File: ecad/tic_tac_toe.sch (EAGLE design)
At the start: 36 parts, among them J1 PJ-102AH, U2 NCP1117ST50T3G, U3 ATMEGA8U2-AU, Y1 ECS-160-12-33-AGN-TR

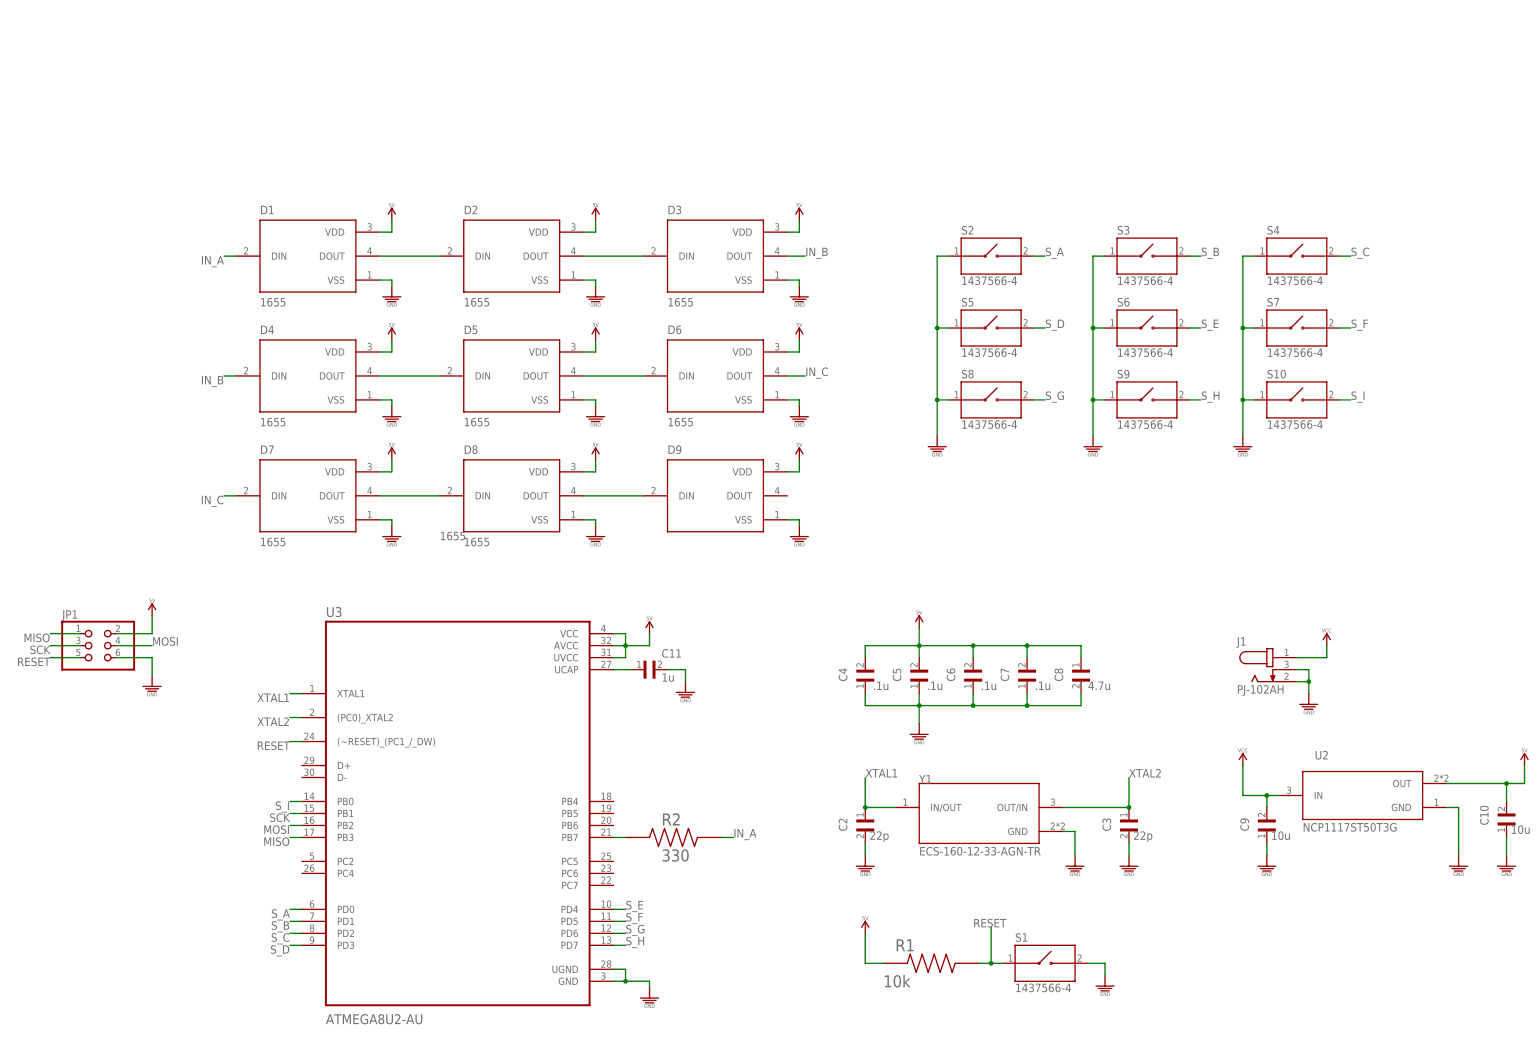
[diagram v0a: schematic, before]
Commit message: ecad, gerbers
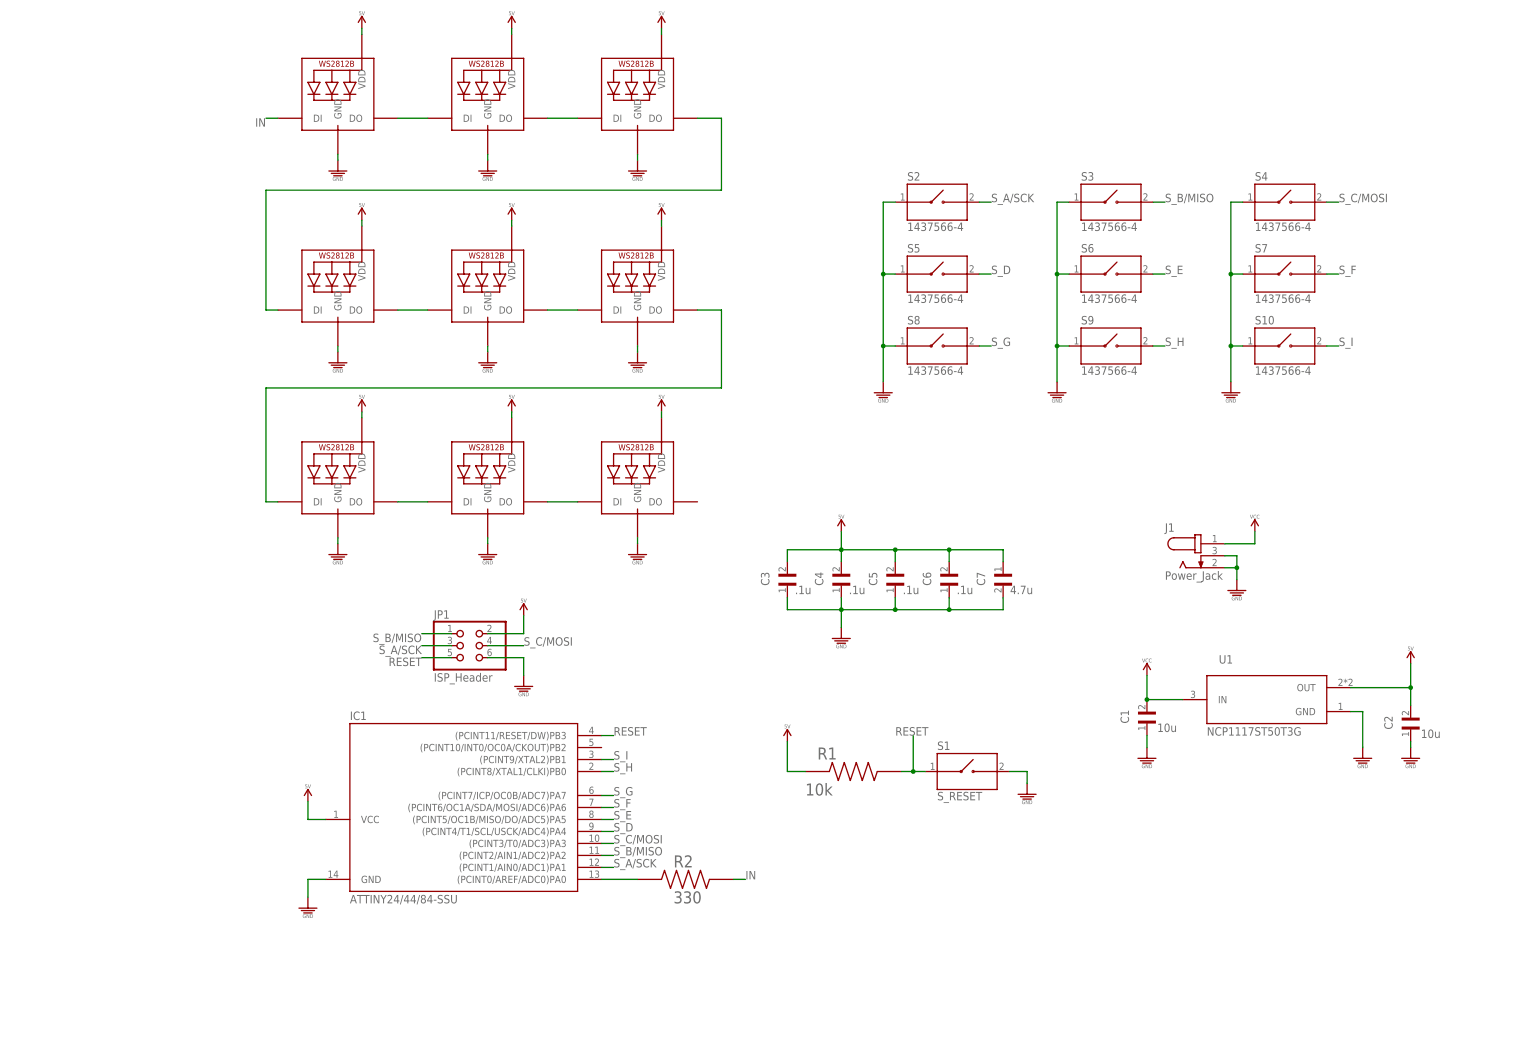
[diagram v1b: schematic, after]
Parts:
- removed C10, C9: 10u, TAJR106M006R:TAJR106M006R
- removed C11: 1u, GRM216R61E105KA12D:GRM216R61E105KA12D
- removed C8: 4.7u, CL21A475KAQNNNE:CL21A475KAQNNNE
- removed D1, D2, D3, D4, D5, D6, D7, D8, D9: 1655, 1655:1655
- removed U2: NCP1117ST50T3G, NCP1117ST50T3G:NCP1117ST50T3G
- removed U3: ATMEGA8U2-AU, ATMEGA8U2-AU:ATMEGA8U2-AU
- removed Y1: ECS-160-12-33-AGN-TR, ECS-160-12-33-AGN-TR:ECS-160-12-33-AGN-TR
- added C1: 10u, TAJR106M006R (1):TAJR106M006R
- added IC1: ATTINY24/44/84-SSU, attiny24_44_84:ATTINY24/44/84-SSU
- added LED1, LED2, LED3, LED4, LED5, LED6, LED7, LED8, LED9: MICROBUILDER_WS2812B_SK6812E, Adafruit Slider Trinkey:MICROBUILDER_WS2812B_SK6812E
- added U1: NCP1117ST50T3G, NCP1117ST50T3G (1):NCP1117ST50T3G
- C2: value 22p -> 10u; device C0805C220J5GACTU:C0805C220J5GACTU -> TAJR106M006R (1):TAJR106M006R
- C3: value 22p -> .1u; device C0805C220J5GACTU:C0805C220J5GACTU -> 08055F104K4T2A:08055F104K4T2A
- C7: value .1u -> 4.7u; device 08055F104K4T2A:08055F104K4T2A -> CL21A475KAQNNNE:CL21A475KAQNNNE
- J1: value PJ-102AH -> Power_Jack
- JP1: value (none) -> ISP_Header
- S1: value 1437566-4 -> S_RESET
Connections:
- removed net IN_A: D1.DIN, R2.2
- removed net IN_B: D3.DOUT, D4.DIN
- removed net IN_C: D6.DOUT, D7.DIN
- removed net MISO: JP1.1, U3.PB3
- removed net MOSI: JP1.4, U3.PB2
- removed net N$1: R2.1, U3.PB7
- removed net N$8: C11.1, U3.UCAP
- removed net SCK: JP1.3, U3.PB1
- removed net S_A: S2.2, U3.PD0
- removed net S_B: S3.2, U3.PD1
- removed net S_C: S4.2, U3.PD2
- removed net XTAL1: C2.1, U3.XTAL1, Y1.IN/OUT
- removed net XTAL2: C3.1, U3.(PC0)_XTAL2, Y1.OUT/IN
- new net IN: LED1.DI, R2.2
- new net N$6: LED7.DO, LED8.DI
- new net N$7: LED8.DO, LED9.DI
- new net N$9: LED3.DO, LED4.DI
- new net S_A/SCK: IC1.(PCINT1/AIN0/ADC1)PA1, JP1.3, S2.2
- new net S_B/MISO: IC1.(PCINT2/AIN1/ADC2)PA2, JP1.1, S3.2
- new net S_C/MOSI: IC1.(PCINT3/T0/ADC3)PA3, JP1.4, S4.2
- net 5V: now also C2.2, C3.2, C7.1, IC1.VCC, LED1.VDD, LED2.VDD, LED3.VDD, LED4.VDD, LED5.VDD, LED6.VDD, LED7.VDD, LED8.VDD, LED9.VDD, U1.OUT; no longer C10.2, C7.2, C8.1, D1.VDD, D2.VDD, D3.VDD, D4.VDD, D5.VDD, D6.VDD, D7.VDD, D8.VDD, D9.VDD, U2.OUT, U3.AVCC, U3.UVCC, U3.VCC
- net GND: now also C1.1, C2.1, C3.1, C7.2, IC1.GND, LED1.GND, LED2.GND, LED3.GND, LED4.GND, LED5.GND, LED6.GND, LED7.GND, LED8.GND, LED9.GND, U1.GND; no longer C10.1, C11.2, C2.2, C3.2, C7.1, C8.2, C9.1, D1.VSS, D2.VSS, D3.VSS, D4.VSS, D5.VSS, D6.VSS, D7.VSS, D8.VSS, D9.VSS, U2.GND, U3.GND, U3.UGND, Y1.GND
- net N$14: now also LED6.DO, LED7.DI; no longer D1.DOUT, D2.DIN
- net N$15: now also IC1.(PCINT0/AREF/ADC0)PA0, R2.1; no longer D7.DOUT, D8.DIN
- net N$2: now also LED1.DO, LED2.DI; no longer D2.DOUT, D3.DIN
- net N$3: now also LED2.DO, LED3.DI; no longer D4.DOUT, D5.DIN
- net N$4: now also LED4.DO, LED5.DI; no longer D5.DOUT, D6.DIN
- net N$5: now also LED5.DO, LED6.DI; no longer D8.DOUT, D9.DIN
- net RESET: now also IC1.(PCINT11/RESET/DW)PB3; no longer U3.(~RESET)_(PC1_/_DW)
- net S_D: now also IC1.(PCINT4/T1/SCL/USCK/ADC4)PA4; no longer U3.PD3
- net S_E: now also IC1.(PCINT5/OC1B/MISO/DO/ADC5)PA5; no longer U3.PD4
- net S_F: now also IC1.(PCINT6/OC1A/SDA/MOSI/ADC6)PA6; no longer U3.PD5
- net S_G: now also IC1.(PCINT7/ICP/OC0B/ADC7)PA7; no longer U3.PD6
- net S_H: now also IC1.(PCINT8/XTAL1/CLKI)PB0; no longer U3.PD7
- net S_I: now also IC1.(PCINT9/XTAL2)PB1; no longer U3.PB0
- net VCC: now also C1.2, U1.IN; no longer C9.2, U2.IN
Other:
- moved on the sheet: C2, C3, C4, C5, C6, C7, J1, JP1, R1, R2, S1, S10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
